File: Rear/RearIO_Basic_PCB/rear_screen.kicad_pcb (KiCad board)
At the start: 2 copper layers, 99.5 x 81.5 mm, 56 parts, among them J1 Conn_01x02_Pin, J2 Conn_01x02_Pin, J3 Conn_01x02_Pin, J4 Conn_01x02_Pin, J5 Conn_01x02_Pin, J6 Conn_01x02_Pin, J7 Conn_01x08_Socket, Q1 NTMFS4C03N-HXY, Q10 MMBT3904, Q2 NTMFS4C03N-HXY, Q3 NTMFS4C03N-HXY, Q4 NTMFS4C03N-HXY, Q5 MMBT3904, Q6 NTMFS4C03N-HXY, Q7 NTMFS4C03N-HXY, Q8 MMBT3904, Q9 MMBT3904, U3 AOZ1280CI, U4 ACS711xEXLT-31AB

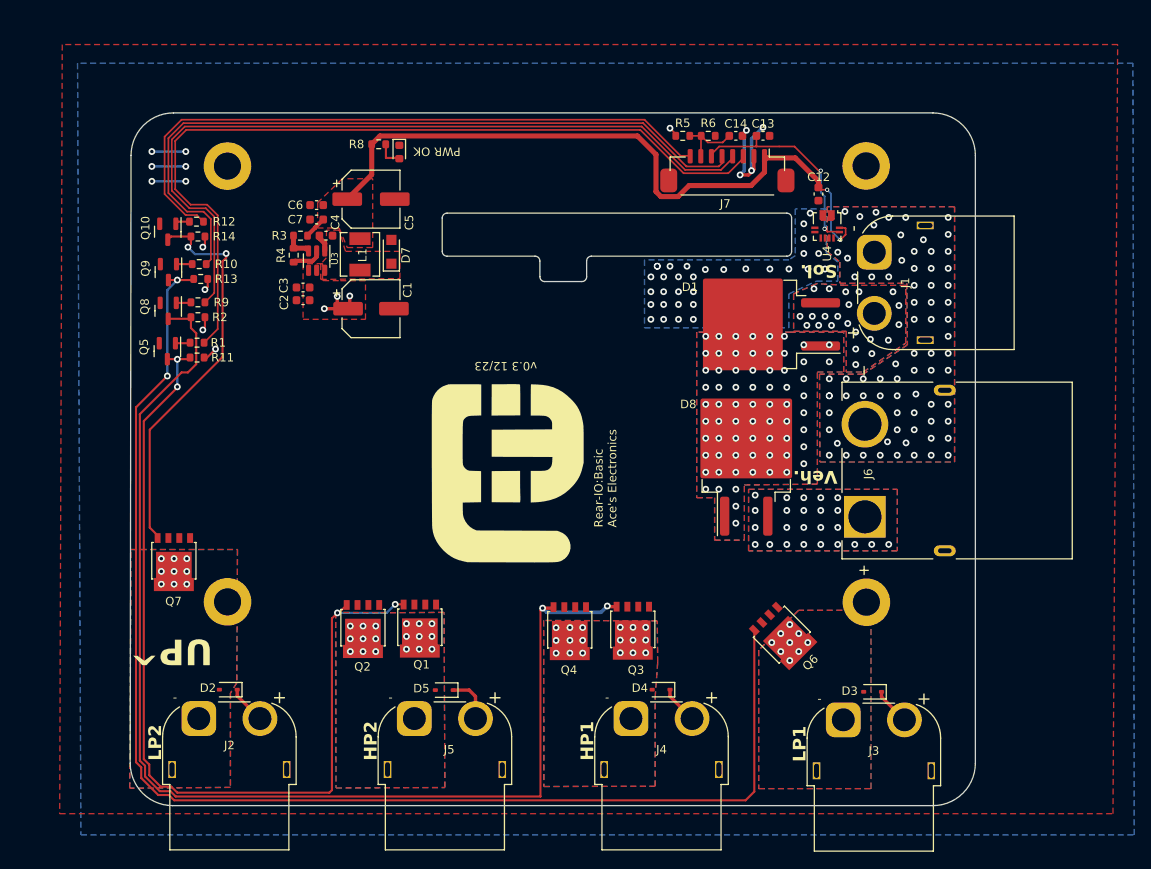
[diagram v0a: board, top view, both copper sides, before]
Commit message: Started work on v0.3 software
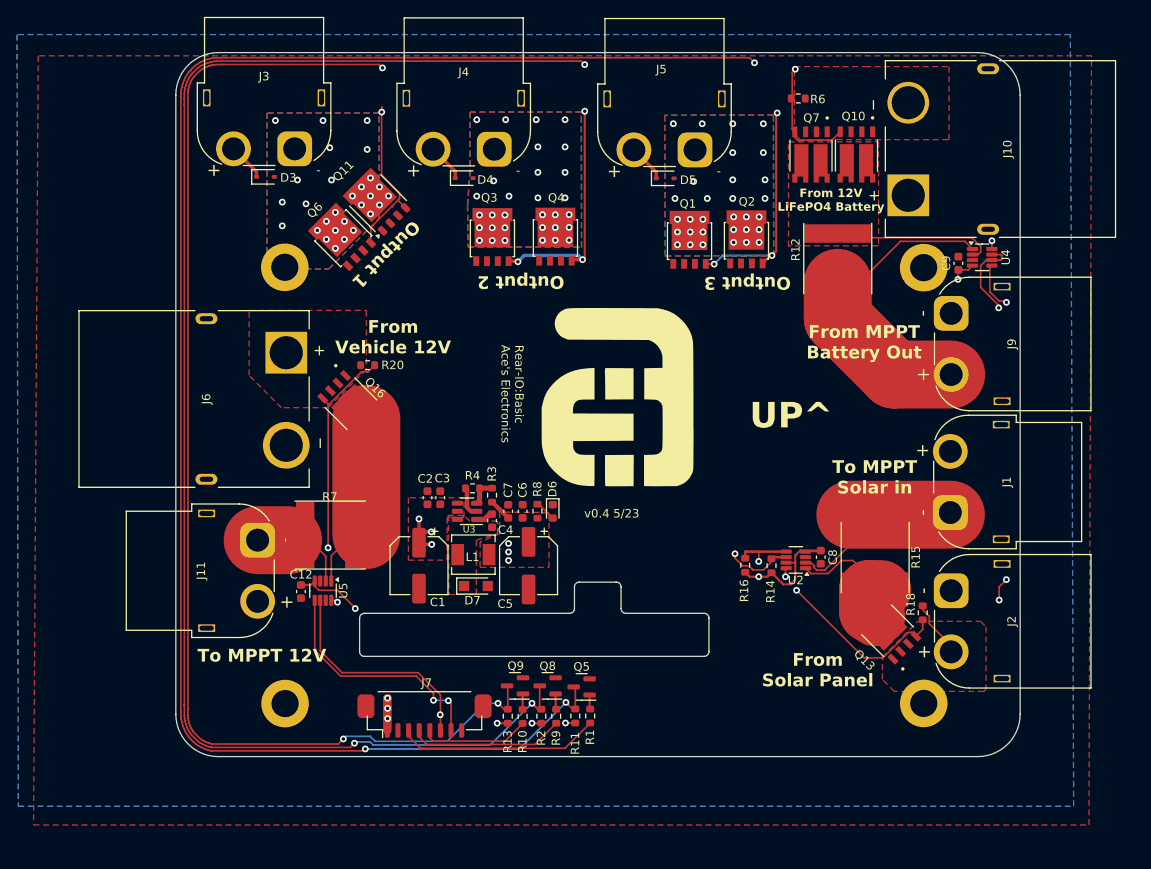
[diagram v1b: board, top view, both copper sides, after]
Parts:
- removed C13, C14: 100nF, Capacitor_SMD:C_0603_1608Metric
- removed D1, D8: CI20S120M3, Package_TO_SOT_SMD:TO-263-2_TabPin1
- removed D2: 1N5819WS, Diode_SMD:D_SOD-323
- removed R5: 82k, Resistor_SMD:R_0603_1608Metric
- added C8: 100nF, Capacitor_SMD:C_0603_1608Metric, F.Cu at (160.0, 114.0)
- added C9: 100nF, Capacitor_SMD:C_0603_1608Metric, F.Cu at (176.2, 79.4)
- added J10: Conn_01x02_Pin, Acea:AMASS_XT90PW-M, F.Cu at (179.7, 66.0)
- added J11: Conn_01x02_Pin, Connector_AMASS:AMASS_XT60PW-F_1x02_P7.20mm_Horizontal, F.Cu at (93.7, 112.0)
- added J9: Conn_01x02_Pin, Connector_AMASS:AMASS_XT60PW-M_1x02_P7.20mm_Horizontal, F.Cu at (175.3, 85.3)
- added Q11: NTMFS4C03N-HXY, Package_TO_SOT_SMD:LFPAK56, F.Cu at (107.9, 72.3)
- added Q13: AON6411, Acea:PowerDI5060-8, F.Cu at (168.0, 122.8)
- added Q16: AON6411, Acea:PowerDI5060-8, F.Cu at (104.6, 95.8)
- added R15: 10mR, Acea:2728R_C500749, F.Cu at (166.4, 114.0)
- added R16: 2k, Resistor_SMD:R_0603_1608Metric, F.Cu at (151.1, 115.0)
- added R18: 16k, Resistor_SMD:R_0603_1608Metric, F.Cu at (172.0, 120.5)
- added R20: 16k, Resistor_SMD:R_0603_1608Metric, F.Cu at (106.7, 91.4)
- added R7: 10mR, Acea:2728R_C500749, F.Cu at (102.2, 111.4)
- added U2: INA236AIDDFR_C5443912, Package_TO_SOT_SMD:SOT-23-8, F.Cu at (157.1, 114.3)
- added U5: INA236AIDDFR_C5443912, Package_TO_SOT_SMD:SOT-23-8, F.Cu at (101.4, 117.9)
- J1: footprint Connector_AMASS:AMASS_XT60PW-M_1x02_P7.20mm_Horizontal -> Connector_AMASS:AMASS_XT60PW-F_1x02_P7.20mm_Horizontal
- J2: footprint Connector_AMASS:AMASS_XT60PW-F_1x02_P7.20mm_Horizontal -> Connector_AMASS:AMASS_XT60PW-M_1x02_P7.20mm_Horizontal
- Q10: value MMBT3904 -> AON6411; footprint Package_TO_SOT_SMD:SOT-23 -> Acea:PowerDI5060-8
- Q7: value NTMFS4C03N-HXY -> AON6411; footprint Package_TO_SOT_SMD:LFPAK56 -> Acea:PowerDI5060-8
- R12: value 1k -> 10mR; footprint Resistor_SMD:R_0603_1608Metric -> Acea:2728R_C500749
- R14: value 16k -> 2k
- U4: value ACS711xEXLT-31AB -> INA236AIDDFR_C5443912; footprint Sensor_Current:Allegro_QFN-12-10-1EP_3x3mm_P0.5mm -> Package_TO_SOT_SMD:SOT-23-8
- moved H1 103.5 mm to (172.1, 131.2), turned to 180 degrees
- moved D3 93.7 mm to (94.6, 69.2), turned to 0 degrees
- moved J3 93.2 mm to (98.1, 65.9), turned to 0 degrees
- moved H2 93.2 mm to (96.9, 131.2), turned to 180 degrees
- moved H4 90.9 mm to (172.1, 79.9), turned to 180 degrees
- moved J2 89.8 mm to (175.3, 118.0), turned to -90 degrees
- moved Q7 89.0 mm to (158.8, 66.6)
- moved J6 87.3 mm to (87.7, 95.4), turned to -90 degrees
- moved Q10 81.6 mm to (164.2, 66.6)
- moved H3 79.0 mm to (96.9, 79.9), turned to 180 degrees
- moved R14 77.9 mm to (154.2, 115.0), turned to -90 degrees
- moved C12 76.8 mm to (98.8, 118.0)
- moved R12 75.6 mm to (162.0, 78.8), turned to -90 degrees
- moved J5 74.7 mm to (145.2, 66.0), turned to 0 degrees
- moved J7 73.0 mm to (113.3, 132.4), turned to 0 degrees
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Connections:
- C1 pad 1: +BATT -> B+
- C2 pad 1: +BATT -> B+
- C3 pad 1: +BATT -> B+
- D3 pad 1: +BATT -> B+
- D4 pad 1: +BATT -> B+
- D5 pad 1: +BATT -> B+
- J1 pad 1: BATT- -> S-
- J1 pad 2: Net-(D1-A) -> GND
- J2 pad 1: Net-(D2-A) -> GND
- J2 pad 2: +BATT -> S
- J3 pad 2: +BATT -> B+
- J4 pad 2: +BATT -> B+
- J5 pad 2: +BATT -> B+
- J6 pad 1: BATT- -> GND
- J6 pad 2: Net-(D8-A) -> V
- Q10 pad 1: Net-(Q10-B) -> B
- Q10 pad 2: GND -> B
- Q10 pad 3: Net-(Q10-C) -> B
- Q7 pad 1: GND -> B
- Q7 pad 2: GND -> B
- Q7 pad 3: GND -> B
- Q7 pad 4: Net-(Q10-C) -> ABFET
- Q7 pad 5: Net-(D2-A) -> B-
- R11 pad 1: +BATT -> B+
- R12 pad 1: GPIO21 -> B-
- R12 pad 2: Net-(Q10-B) -> B+
- R13 pad 1: +BATT -> B+
- R14 pad 1: +BATT -> GPIO13
- R14 pad 2: Net-(Q10-C) -> +5V
- R2 pad 1: +BATT -> B+
- R6 pad 1: GPIO14 -> B
- R6 pad 2: GND -> ABFET
- U3 pad 4: +BATT -> B+
- U3 pad 5: +BATT -> B+
- U4 pad 1: BATT- -> B+
- U4 pad 2: GND -> B-
- U4 pad 4: unconnected-(U4-~{FAULT}-Pad4) -> +5V
- U4 pad 5: unconnected-(U4-NC-Pad5) -> GPIO14
- U4 pad 6: unconnected-(U4-NC-Pad6) -> GPIO13
- U4 pad 7: unconnected-(U4-NC-Pad7) -> GPIO13
- U4 pad 8: unconnected-(U4-NC-Pad8) -> ABFET
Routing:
- net GPIO14: track 7.39 -> 199.8 mm, vias 0 -> 6
- net GPIO13: track 24.7 -> 201.4 mm, vias 2 -> 3
- net Net-(Q1-G): track 107.0 -> 232.6 mm, vias 4 -> 6
- net +5V: track 83.9 -> 192.3 mm, vias 2 -> 9
- net GPIO21: track 77.2 -> 0.00 mm
- net GPIO12: track 87.3 -> 13.0 mm
- net GPIO10: track 98.1 -> 23.9 mm
- net GPIO11: track 92.4 -> 18.3 mm
- net Net-(Q3-G): track 140.9 -> 206.0 mm, vias 2 -> 6
- net B+: track 0.00 -> 61.6 mm, vias 0 -> 6
- net ABFET: track 0.00 -> 58.9 mm, vias 0 -> 2
- net Net-(Q10-C): track 46.8 -> 0.00 mm, vias 2 -> 0
- net AVFET: track 0.00 -> 32.9 mm, vias 0 -> 2
- net +BATT: track 32.8 -> 0.00 mm, vias 77 -> 0
- net GND: track 31.2 -> 3.66 mm, vias 42 -> 0
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- added copper zone on F.Cu, net B
- added copper zone on B.Cu, net B+
- added copper zone on F.Cu, net B+
- added copper zone on In2.Cu, net B+
- added copper zone on F.Cu, net B-
- added copper zone on In1.Cu, net GND
- added copper zone on In1.Cu, net Net-(D3-A)
- added copper zone on In2.Cu, net Net-(D3-A)
- added copper zone on In1.Cu, net Net-(D4-A)
- added copper zone on In2.Cu, net Net-(D4-A)
- added copper zone on In1.Cu, net Net-(D5-A)
- added copper zone on In2.Cu, net Net-(D5-A)
- added copper zone on F.Cu, net S
- added copper zone on F.Cu, net V
- removed copper zone on B.Cu, net +BATT
- removed copper zone on F.Cu, net +BATT
- removed copper zone on B.Cu, net BATT-
- removed copper zone on F.Cu, net BATT-
- removed copper zone on B.Cu, net GND
- removed copper zone on B.Cu, net Net-(D1-A)
- removed copper zone on F.Cu, net Net-(D1-A)
- removed copper zone on B.Cu, net Net-(D2-A)
- removed copper zone on F.Cu, net Net-(D2-A)
- removed copper zone on B.Cu, net Net-(D8-A)
- removed copper zone on F.Cu, net Net-(D8-A)
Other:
- board size 99.5 x 81.5 mm -> 99.4 x 82.9 mm
- copper layers 2 -> 4
- board text added: "From 12V LiFePO4 Battery"
- board text added: "From MPPT Battery Out"
- board text added: "From Solar Panel"
- board text added: "From Vehicle 12V"
- board text added: "Output 1"
- board text added: "Output 2"
- board text added: "Output 3"
- board text added: "To MPPT 12V"
- board text added: "To MPPT Solar in"
- board text added: "v0.4 5/23"
- board text removed: "HP1"
- board text removed: "HP2"
- board text removed: "LP1"
- board text removed: "LP2"
- board text removed: "PWR OK"
- board text removed: "Sol."
- board text removed: "Veh."
- board text removed: "v0.3 12/23"
